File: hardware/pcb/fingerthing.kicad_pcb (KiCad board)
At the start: 2 copper layers, 52 x 51 mm, 43 parts, among them J1 10103594-0001LF, J2 TSW-118-07-L-D, J3 TSW-118-07-L-D, J4 SM03B-SRSS-TB(LF)(SN), SW1 434133025816, SW2 434133025816, U1 RP2350A, U2 NCP1117ST33T3G, U3 W25Q128JVSIQ, X1 12MHz

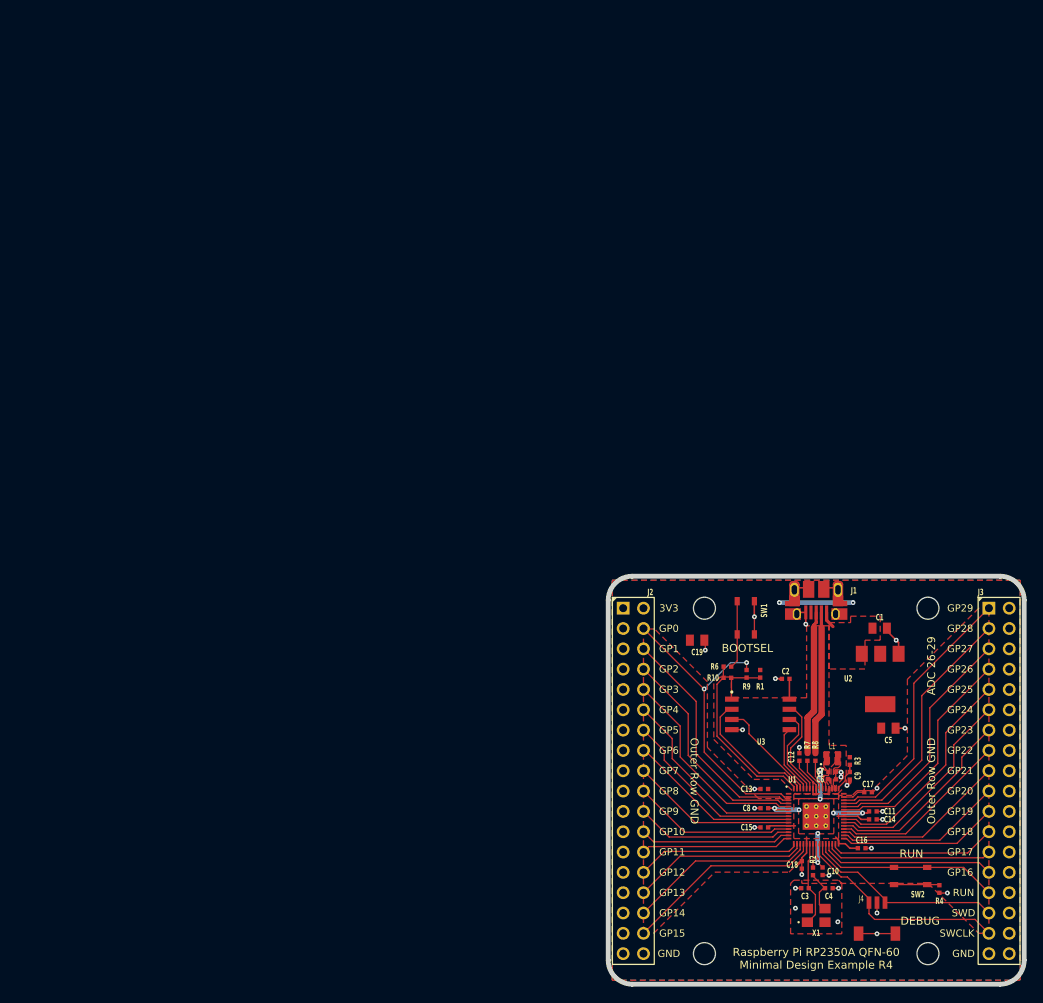
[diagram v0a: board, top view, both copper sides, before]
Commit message: usb / sensor layout
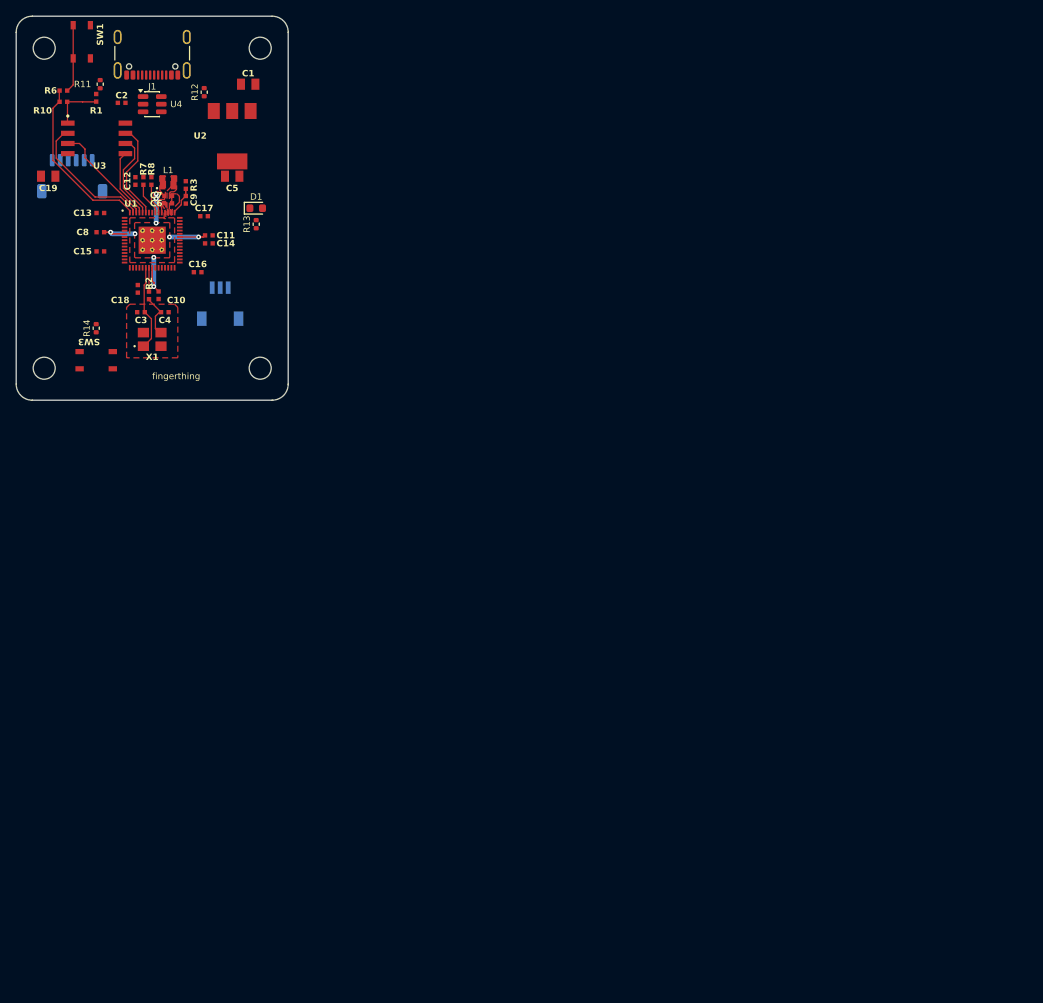
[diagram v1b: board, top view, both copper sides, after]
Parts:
- removed J3: TSW-118-07-L-D, RPI_COMPILED:samtec_tsw-118-07-l-d
- removed R4: 1k, RPI_COMPILED:generic_resc1005x35
- removed R9: 0, RPI_COMPILED:generic_resc1005x35
- removed SW2: 434133025816, RPI_COMPILED:wurthelek_434133025816
- added D1: green, LED_SMD:LED_0603_1608Metric, F.Cu at (30.0, 24.0)
- added R11: 5.1k, Resistor_SMD:R_0402_1005Metric, F.Cu at (10.5, 8.50)
- added R12: 5.1k, Resistor_SMD:R_0402_1005Metric, F.Cu at (23.5, 9.50)
- added R13: 1k, Resistor_SMD:R_0402_1005Metric, F.Cu at (30.0, 26.0)
- added R14: 10k, Resistor_SMD:R_0402_1005Metric, F.Cu at (10.0, 39.0)
- added SW3: 434133025816, RPI_COMPILED:wurthelek_434133025816, F.Cu at (10.0, 43.0)
- added U4: USBLC6-2SC6, Package_TO_SOT_SMD:SOT-23-6, F.Cu at (17.0, 11.0)
- J1: value 10103594-0001LF -> USB4105-GF-A; footprint RPI_COMPILED:amphenol_10103594-0001lf -> Connector_USB:USB_C_Receptacle_GCT_USB4105-xx-A_16P_TopMnt_Horizontal
- J2: value TSW-118-07-L-D -> R503; footprint RPI_COMPILED:samtec_tsw-118-07-l-d -> Connector_JST:JST_SH_SM06B-SRSS-TB_1x06-1MP_P1.00mm_Horizontal; moved to B.Cu
- J4: moved to B.Cu
- moved J4 112.5 mm to (25.5, 38.5), turned to 180 degrees
- moved MH3 111.0 mm to (30.5, 44.0)
- moved MH4 110.3 mm to (3.50, 44.0)
- moved C10 109.9 mm to (17.8, 34.9)
- moved C11 109.9 mm to (24.1, 27.4)
- moved C12 109.9 mm to (14.9, 20.6)
- moved C13 109.9 mm to (10.5, 24.6)
- moved C14 109.9 mm to (24.1, 28.4)
- moved C15 109.9 mm to (10.5, 29.4)
- moved C16 109.9 mm to (22.7, 32.0)
- moved C17 109.9 mm to (23.5, 25.0)
- moved C18 109.9 mm to (15.2, 34.1)
- moved C2 109.9 mm to (13.2, 10.8)
- moved C3 109.9 mm to (15.6, 37.0)
- moved C4 109.9 mm to (18.6, 37.0)
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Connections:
- net +1V1 renamed /+1V1
- net Net-(U1-USB_DM) renamed /USB_DM
- net Net-(U1-USB_DP) renamed /USB_DP
- C1 pad 1: VBUS -> /VBUS
- C1 pad 2: GND -> /GND
- C10 pad 2: GND -> /GND
- C11 pad 2: GND -> /GND
- C12 pad 1: +3V3 -> /+3V3
- C12 pad 2: GND -> /GND
- C13 pad 1: +3V3 -> /+3V3
- C13 pad 2: GND -> /GND
- C14 pad 1: +3V3 -> /+3V3
- C14 pad 2: GND -> /GND
- C15 pad 1: +3V3 -> /+3V3
- C15 pad 2: GND -> /GND
- C16 pad 1: +3V3 -> /+3V3
- C16 pad 2: GND -> /GND
- C17 pad 1: +3V3 -> /+3V3
- C17 pad 2: GND -> /GND
- C18 pad 1: +3V3 -> /+3V3
- C18 pad 2: GND -> /GND
- C19 pad 1: +3V3 -> /+3V3
- C19 pad 2: GND -> /GND
- C2 pad 1: +3V3 -> /+3V3
- C2 pad 2: GND -> /GND
- C3 pad 2: GND -> /GND
- C4 pad 2: GND -> /GND
- C5 pad 1: +3V3 -> /+3V3
- C5 pad 2: GND -> /GND
- C6 pad 1: +3V3 -> /+3V3
- C6 pad 2: GND -> /GND
- C7 pad 2: GND -> /GND
- C8 pad 2: GND -> /GND
- C9 pad 2: GND -> /GND
- J2 pad 1: GND -> /+3V3
- J2 pad 2: +3V3 -> /GND
- J2 pad 3: GND -> /GPIO5
- J2 pad 4: /GPIO0 -> /GPIO4
- J2 pad 5: GND -> /GPIO7
- J2 pad 6: /GPIO1 -> /+3V3
- J4 pad 2: GND -> /GND
- J4 pad 4: GND -> /GND
- J4 pad 5: GND -> /GND
- R1 pad 1: +3V3 -> /+3V3
- R3 pad 1: +3V3 -> /+3V3
- SW1 pad 1: GND -> /GND
- SW1 pad 2: GND -> /GND
- U1 pad 1: +3V3 -> /+3V3
- U1 pad 11: +3V3 -> /+3V3
- U1 pad 12: /GPIO8 -> unconnected-(U1-GPIO8-Pad12)
- U1 pad 13: /GPIO9 -> unconnected-(U1-GPIO9-Pad13)
- U1 pad 14: /GPIO10 -> unconnected-(U1-GPIO10-Pad14)
- U1 pad 15: /GPIO11 -> unconnected-(U1-GPIO11-Pad15)
- U1 pad 16: /GPIO12 -> unconnected-(U1-GPIO12-Pad16)
- U1 pad 17: /GPIO13 -> unconnected-(U1-GPIO13-Pad17)
- U1 pad 18: /GPIO14 -> unconnected-(U1-GPIO14-Pad18)
- U1 pad 19: /GPIO15 -> unconnected-(U1-GPIO15-Pad19)
- U1 pad 2: /GPIO0 -> unconnected-(U1-GPIO0-Pad2)
- U1 pad 20: +3V3 -> /+3V3
- U1 pad 26: /RUN -> unconnected-(U1-RUN-Pad26)
- U1 pad 27: /GPIO16 -> unconnected-(U1-GPIO16-Pad27)
- U1 pad 28: /GPIO17 -> unconnected-(U1-GPIO17-Pad28)
- U1 pad 29: /GPIO18 -> unconnected-(U1-GPIO18-Pad29)
- U1 pad 3: /GPIO1 -> unconnected-(U1-GPIO1-Pad3)
- U1 pad 30: +3V3 -> /+3V3
- U1 pad 31: /GPIO19 -> unconnected-(U1-GPIO19-Pad31)
- U1 pad 32: /GPIO20 -> unconnected-(U1-GPIO20-Pad32)
- U1 pad 33: /GPIO21 -> unconnected-(U1-GPIO21-Pad33)
- U1 pad 34: /GPIO22 -> unconnected-(U1-GPIO22-Pad34)
- U1 pad 35: /GPIO23 -> unconnected-(U1-GPIO23-Pad35)
- U1 pad 36: /GPIO24 -> unconnected-(U1-GPIO24-Pad36)
- U1 pad 38: +3V3 -> /+3V3
- U1 pad 4: /GPIO2 -> unconnected-(U1-GPIO2-Pad4)
- U1 pad 40: /GPIO26_ADC0 -> unconnected-(U1-GPIO26_ADC0-Pad40)
- U1 pad 41: /GPIO27_ADC1 -> unconnected-(U1-GPIO27_ADC1-Pad41)
- U1 pad 42: /GPIO28_ADC2 -> unconnected-(U1-GPIO28_ADC2-Pad42)
- U1 pad 43: /GPIO29_ADC3 -> unconnected-(U1-GPIO29_ADC3-Pad43)
- U1 pad 44: +3V3 -> /+3V3
- U1 pad 45: +3V3 -> /+3V3
- U1 pad 47: GND -> /GND
- U1 pad 49: +3V3 -> /+3V3
- U1 pad 5: /GPIO3 -> unconnected-(U1-GPIO3-Pad5)
- U1 pad 53: +3V3 -> /+3V3
- U1 pad 54: +3V3 -> /+3V3
- U1 pad 61: GND -> /GND
- U2 pad 1: GND -> /GND
- U2 pad 2: +3V3 -> /+3V3
- U2 pad 3: VBUS -> /VBUS
- U2 pad 4: +3V3 -> /+3V3
- U3 pad 4: GND -> /GND
- U3 pad 8: +3V3 -> /+3V3
- X1 pad 2: GND -> /GND
- X1 pad 4: GND -> /GND
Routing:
- net /GPIO0: track 39.0 -> 0.00 mm, vias 2 -> 0
- net +3V3: track 37.6 -> 0.00 mm, vias 2 -> 0
- net GND: track 37.5 -> 0.00 mm, vias 27 -> 0
- net /GPIO29_ADC3: track 33.6 -> 0.00 mm
- net /GPIO28_ADC2: track 31.9 -> 0.00 mm
- net /GPIO27_ADC1: track 30.3 -> 0.00 mm
- net /GPIO1: track 29.8 -> 0.00 mm
- net /GPIO26_ADC0: track 28.6 -> 0.00 mm
- net /GPIO2: track 28.2 -> 0.00 mm
- net /SWCLK: track 27.8 -> 0.00 mm
- net /GPIO25: track 27.7 -> 0.00 mm
- net /GPIO3: track 26.5 -> 0.00 mm
- net /GPIO24: track 26.1 -> 0.00 mm
- net /SWD: track 25.4 -> 0.00 mm
- net /GPIO15: track 25.2 -> 0.00 mm
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- added copper zone on F.Cu, net /+3V3
- added copper zone on F.Cu, net /GND
- removed copper zone on F.Cu, net +3V3
- removed copper zone on B.Cu, net GND
- removed copper zone on F.Cu, net GND
- removed copper zone on F.Cu, net VBUS
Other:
- board size 52 x 51 mm -> 34 x 48 mm
- copper layers 2 -> 4
- board text added: "CLK GND SWD"
- board text added: "fingerthing"
- board text removed: "3V3"
- board text removed: "ADC 26-29"
- board text removed: "BOOTSEL"
- board text removed: "DEBUG"
- board text removed: "GND"
- board text removed: "GP0"
- board text removed: "GP1"
- board text removed: "GP10"
- board text removed: "GP11"
- board text removed: "GP12"
- board text removed: "GP13"
- board text removed: "GP14"
- board text removed: "GP15"
- board text removed: "GP16"
- board text removed: "GP17"
- board text removed: "GP18"
- board text removed: "GP19"
- board text removed: "GP2"
- board text removed: "GP20"
- board text removed: "GP21"
- board text removed: "GP22"
- board text removed: "GP23"
- board text removed: "GP24"
- board text removed: "GP25"
- board text removed: "GP26"
- board text removed: "GP27"
- board text removed: "GP28"
- board text removed: "GP29"
- board text removed: "GP3"
- board text removed: "GP4"
- board text removed: "GP5"
- board text removed: "GP6"
- board text removed: "GP7"
- board text removed: "GP8"
- board text removed: "GP9"
- board text removed: "Minimal Design Example R4"
- board text removed: "Outer Row GND"
- board text removed: "RUN"
- board text removed: "Raspberry Pi RP2350A QFN-60"
- board text removed: "SWCLK"
- board text removed: "SWD"
